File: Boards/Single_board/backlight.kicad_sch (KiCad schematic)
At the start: 38 parts

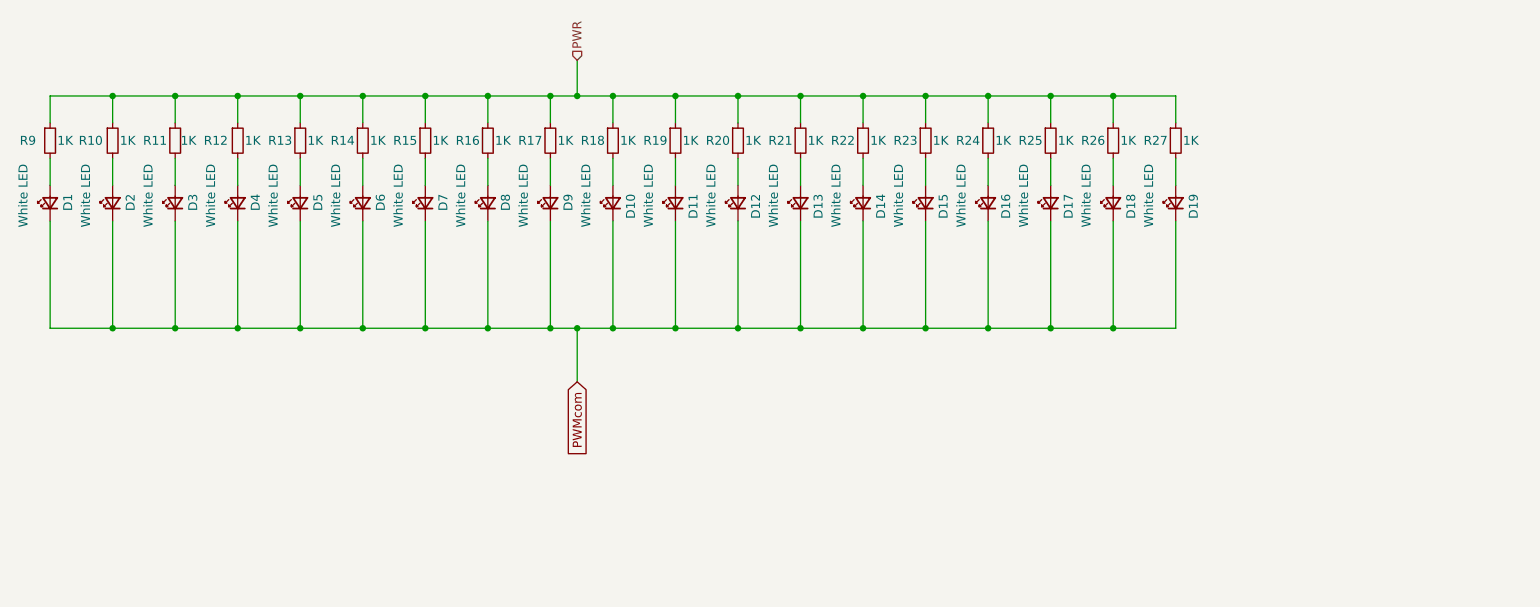
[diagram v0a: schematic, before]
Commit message: some progress on the arduino boilerplate
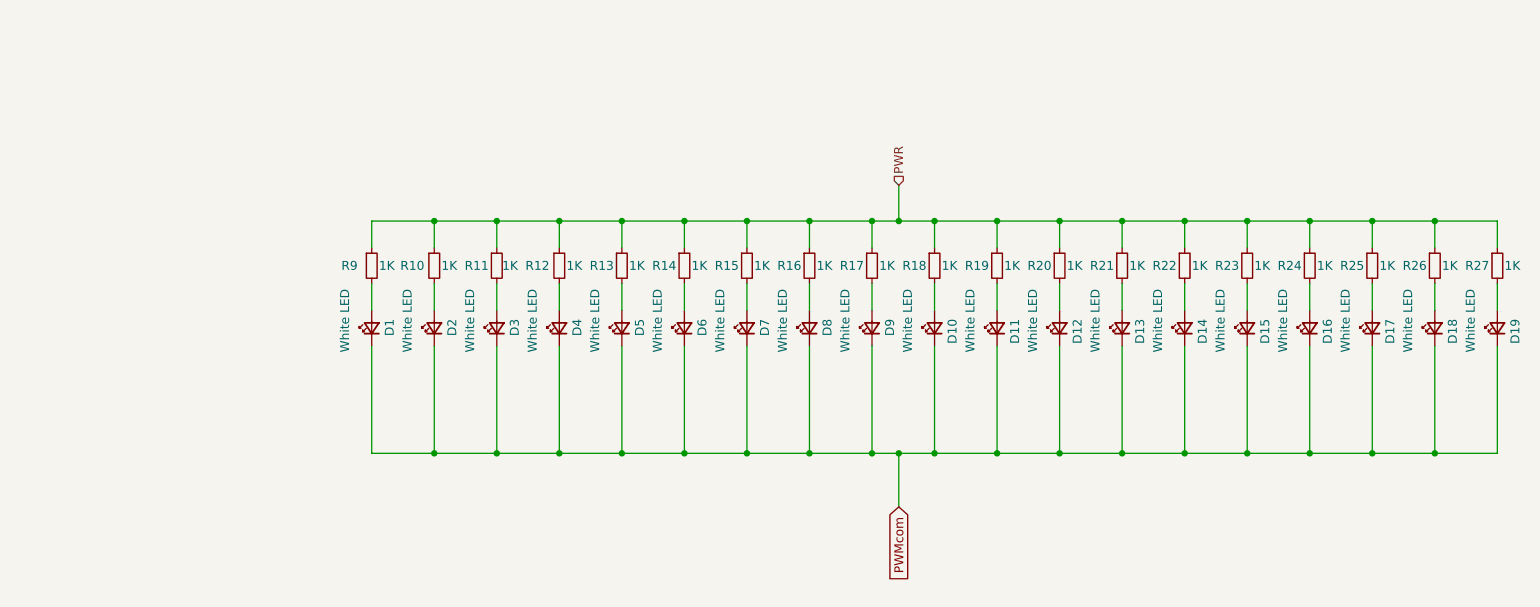
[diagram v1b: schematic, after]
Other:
- company: (none) -> Pablo Ortiz López, Evan MacDonald
- title: (none) -> Backlight for DSKY Keyboard
- moved on the sheet: D1, D10, D11, D12, D13, D14, D15, D16, D17, D18, D19, D2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
